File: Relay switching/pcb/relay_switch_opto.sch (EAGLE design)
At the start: 12 parts, among them K1 G5V-2, Q1 2N3904, SW1 MOMENTARY, U1 ATTINY85-20P

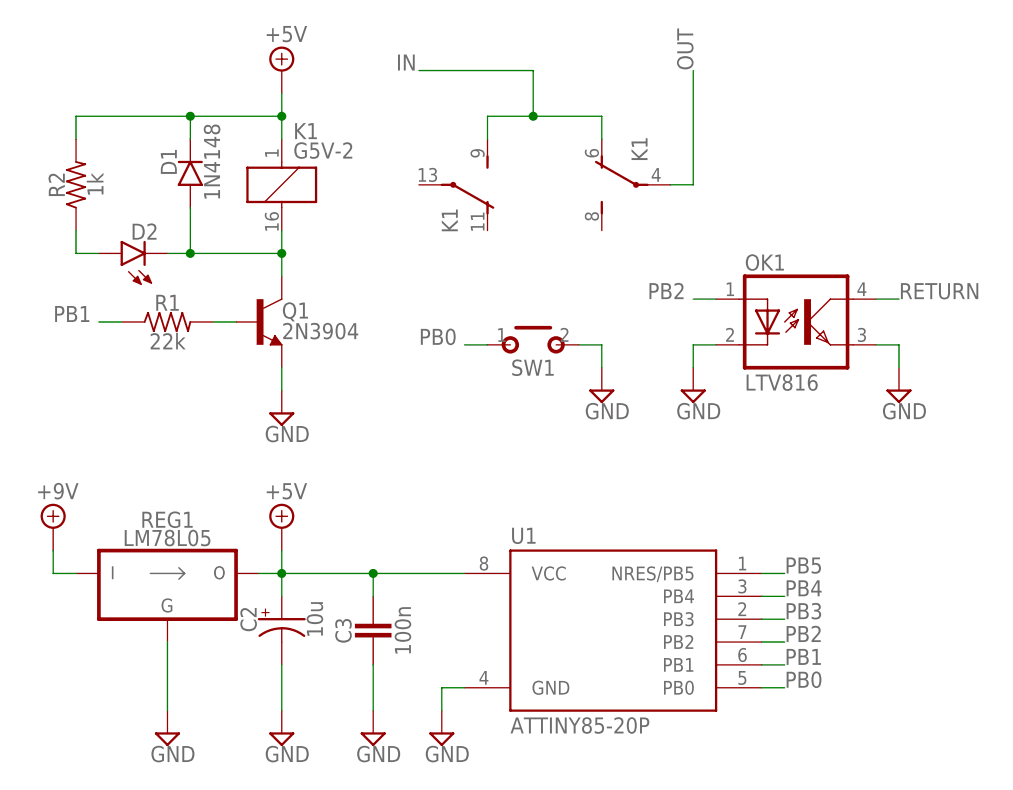
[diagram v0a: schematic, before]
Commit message: 20181201
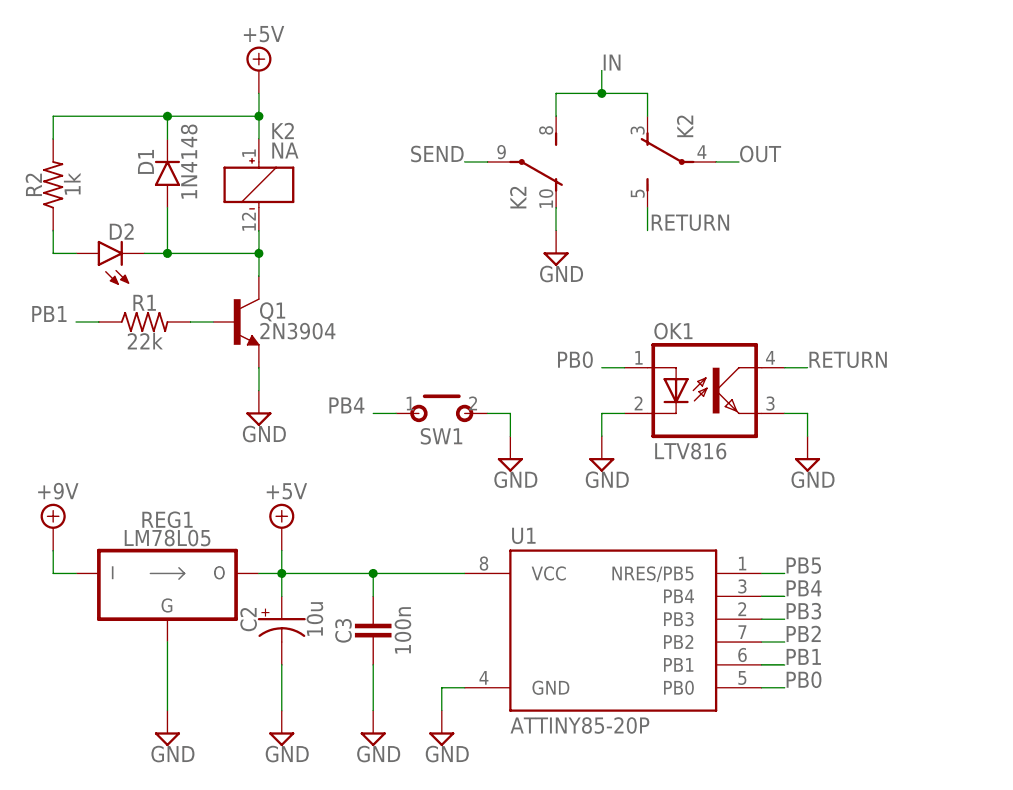
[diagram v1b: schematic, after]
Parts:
- removed K1: G5V-2, pedals-relays:G5V-2
- added K2: NA, pedals-relays:NA
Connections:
- new net SEND: K23.P
- net +5V: now also K21.+; no longer K1A.1
- net GND: now also K23.O
- net IN: now also K22.O, K23.S; no longer K11.O, K12.S
- net N$2: now also K21.-; no longer K1A.2
- net OUT: now also K22.P; no longer K11.P
- net PB0: now also OK1.A; no longer SW1.P
- net PB2: no longer OK1.A
- net PB4: now also SW1.P
- net RETURN: now also K22.S
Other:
- moved on the sheet: D1, D2, OK1, Q1, R1, R2, SW1
